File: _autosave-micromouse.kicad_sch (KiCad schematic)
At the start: 15 parts, among them J1 XT60-M, SW1 SW_SPST, SW2 SW_Push, SW3 SW_SPDT_312, SW4 SW_Push, U1 BUCK, U2 STM32 Blackpill, U3 N20 encoder right, U4 N20 encoder left, U5 TB6612FNG, U6 VL53L0X left, U7 VL53L0X right, U8 VL53L0X middle, U9 oled i2c

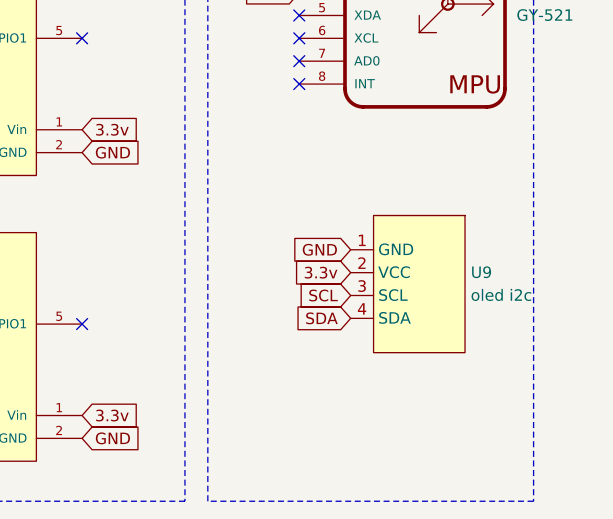
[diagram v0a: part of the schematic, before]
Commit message: pcb changes
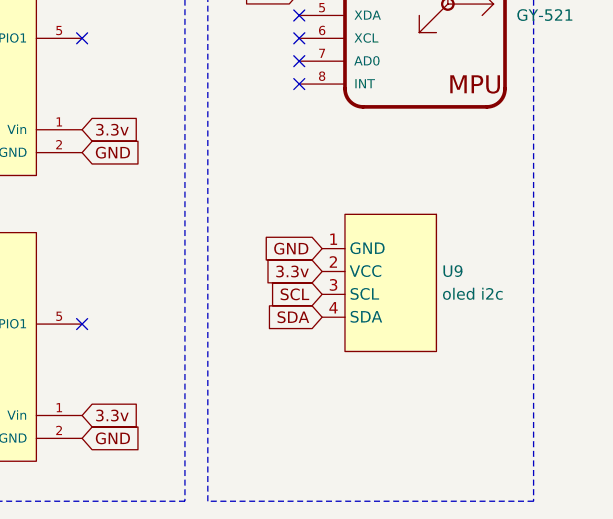
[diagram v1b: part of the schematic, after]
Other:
- moved on the sheet: U9
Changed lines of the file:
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@@
 	(global_label "SDA"
 		(shape input)
-		(at 259.715 121.285 180)
+		(at 256.54 121.158 180)
 		(fields_autoplaced yes)
 		(effects
@@
 		)
 		(property "Intersheetrefs" "${INTERSHEET_REFS}"
-			(at 253.1617 121.285 0)
+			(at 249.9867 121.158 0)
 			(effects
 				(font
@@
 	(global_label "SCL"
 		(shape input)
-		(at 259.715 118.745 180)
+		(at 256.54 118.618 180)
 		(fields_autoplaced yes)
 		(effects
@@
 		)
 		(property "Intersheetrefs" "${INTERSHEET_REFS}"
-			(at 253.2222 118.745 0)
+			(at 250.0472 118.618 0)
 			(effects
 				(font
@@
 	(global_label "3.3v"
 		(shape input)
-		(at 259.715 116.205 180)
+		(at 256.54 116.078 180)
 		(fields_autoplaced yes)
 		(effects
@@
 		)
 		(property "Intersheetrefs" "${INTERSHEET_REFS}"
-			(at 252.7384 116.205 0)
+			(at 249.5634 116.078 0)
 			(effects
 				(font
@@
 	(global_label "GND"
 		(shape input)
-		(at 259.715 113.665 180)
+		(at 256.54 113.538 180)
 		(fields_autoplaced yes)
 		(effects
@@
 		)
 		(property "Intersheetrefs" "${INTERSHEET_REFS}"
-			(at 252.8593 113.665 0)
+			(at 249.6843 113.538 0)
 			(effects
 				(font
@@
 	(symbol
 		(lib_id "Screen_oled:Oled")
-		(at 267.335 117.475 270)
+		(at 264.16 117.348 270)
 		(unit 1)
 		(exclude_from_sim no)
@@
 		(fields_autoplaced yes)
 		(property "Reference" "U9"
-			(at 273.05 116.2049 90)
+			(at 269.875 116.0779 90)
 			(effects
 				(font
@@
 		)
 		(property "Value" "oled i2c"
-			(at 273.05 118.7449 90)
+			(at 269.875 118.6179 90)
 			(effects
 				(font
@@
 		)
 		(property "Footprint" "oled:oled"
-			(at 263.525 114.935 0)
+			(at 260.35 114.808 0)
 			(effects
 				(font
@@
 		)
 		(property "Datasheet" ""
-			(at 263.525 114.935 0)
+			(at 260.35 114.808 0)
 			(effects
 				(font
@@
 		)
 		(property "Description" ""
-			(at 263.525 114.935 0)
-			(effects
-				(font
+			(at 260.35 114.808 0)
+			(effects
+				(font
